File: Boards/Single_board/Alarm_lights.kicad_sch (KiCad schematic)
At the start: 46 parts, among them Q1 SI2306, Q10 SI2306, Q11 SI2306, Q12 SI2306, Q13 SI2306, Q14 SI2306, Q2 SI2306, Q3 SI2306, Q4 SI2306, Q5 SI2306, Q6 SI2306, Q7 SI2306, Q8 SI2306, Q9 SI2306, U1 PCF8575

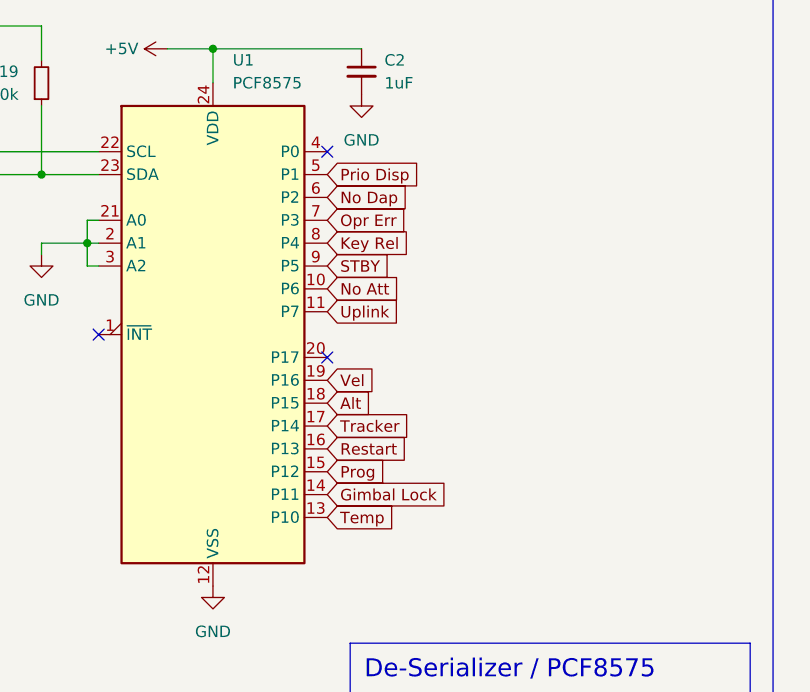
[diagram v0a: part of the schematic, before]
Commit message: some progress on the arduino boilerplate
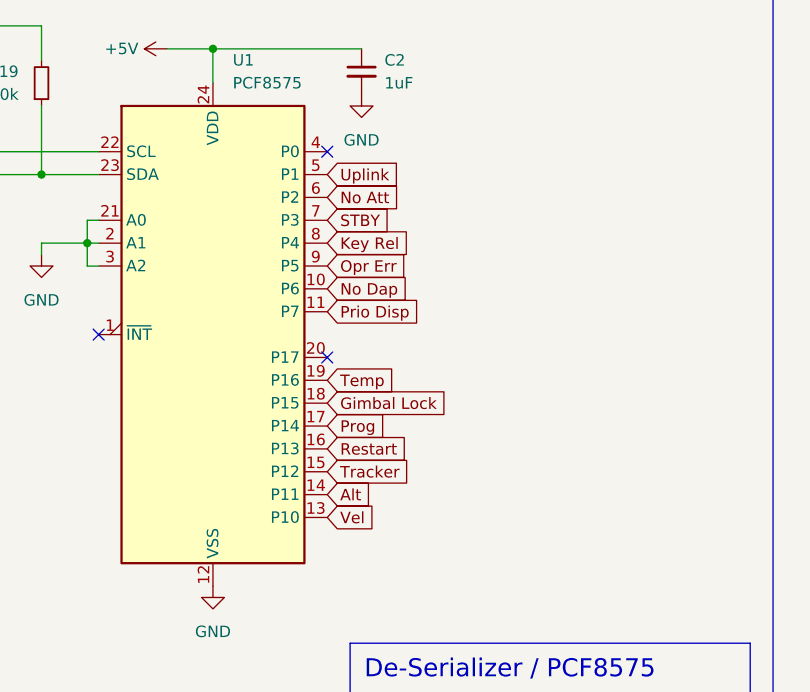
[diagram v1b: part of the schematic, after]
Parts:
- C2: footprint Capacitor_SMD:C_1206_3216Metric_Pad1.33x1.80mm_HandSolder -> Capacitor_SMD:C_0805_2012Metric
- D1, D10, D11, D12, D13, D14, D2, D3, D4, D5, D6, D7, D8, D9: footprint LED_SMD:LED_1206_3216Metric_Pad1.42x1.75mm_HandSolder -> LED_SMD:LED_1206_3216Metric
- Q1, Q10, Q11, Q12, Q13, Q14, Q2, Q3, Q4, Q5, Q6, Q7, Q8, Q9: footprint Package_TO_SOT_SMD:SOT-23-3 -> Package_TO_SOT_SMD:SOT-23
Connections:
- net Alt: now also U1.14 (P11); no longer U1.18 (P15)
- net Gimbal Lock: now also U1.18 (P15); no longer U1.14 (P11)
- net No Att: now also U1.6 (P2); no longer U1.10 (P6)
- net No Dap: now also U1.10 (P6); no longer U1.6 (P2)
- net Opr Err: now also U1.9 (P5); no longer U1.7 (P3)
- net Prio Disp: now also U1.11 (P7); no longer U1.5 (P1)
- net Prog: now also U1.17 (P14); no longer U1.15 (P12)
- net STBY: now also U1.7 (P3); no longer U1.9 (P5)
- net Temp: now also U1.19 (P16); no longer U1.13 (P10)
- net Tracker: now also U1.15 (P12); no longer U1.17 (P14)
- net Uplink: now also U1.5 (P1); no longer U1.11 (P7)
- net Vel: now also U1.13 (P10); no longer U1.19 (P16)
